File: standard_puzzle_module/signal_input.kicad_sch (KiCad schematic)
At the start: 6 parts

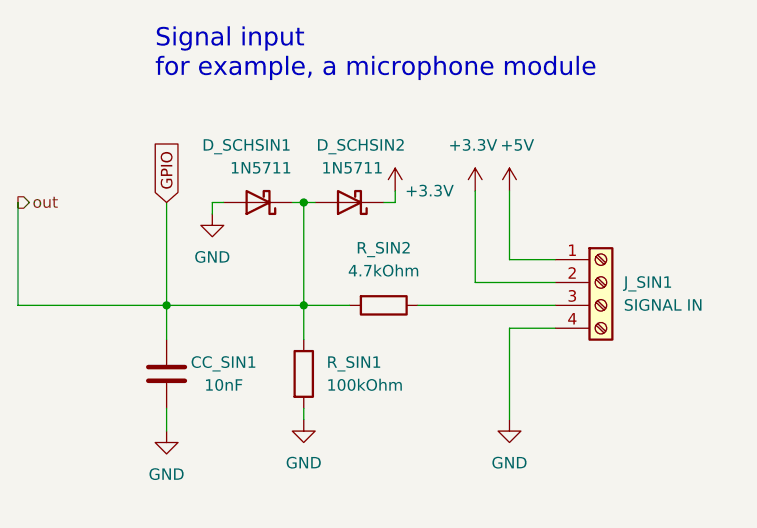
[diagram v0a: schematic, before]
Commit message: feat: dump working files before blackout
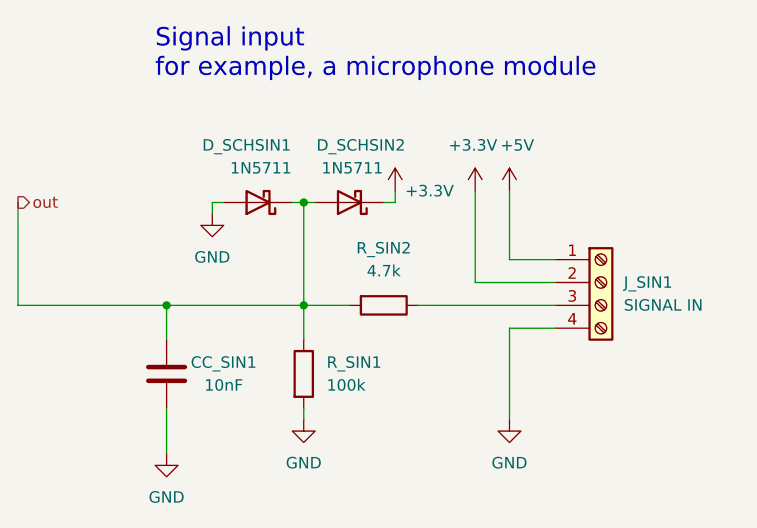
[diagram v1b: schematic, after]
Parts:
- R_SIN1: value 100kOhm -> 100k
- R_SIN2: value 4.7kOhm -> 4.7k
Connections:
- net GPIO renamed out
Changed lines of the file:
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@@
 	(wire
 		(pts
-			(xy 119.38 96.52) (xy 119.38 107.95)
+			(xy 119.38 119.38) (xy 119.38 124.46)
 		)
 		(stroke
@@
 	(wire
 		(pts
-			(xy 119.38 119.38) (xy 119.38 121.92)
-		)
-		(stroke
-			(width 0)
-			(type default)
-		)
-	)
-	(wire
-		(pts
 			(xy 157.48 110.49) (xy 157.48 120.65)
 		)
@@
 			(width 0)
 			(type default)
-		)
-	)
-	(global_label "GPIO"
-		(shape input)
-		(at 119.38 96.52 90)
-		(fields_autoplaced yes)
-		(effects
-			(font
-				(size 1.27 1.27)
-			)
-			(justify left)
-		)
-		(property "Intersheetrefs" "${INTERSHEET_REFS}"
-			(at 119.38 89.0595 90)
-			(hide yes)
-			(show_name no)
-			(do_not_autoplace no)
-			(effects
-				(font
-					(size 1.27 1.27)
-				)
-				(justify left)
-			)
 		)
 	)
@@
 			)
 		)
-		(property "Value" "4.7kOhm"
+		(property "Value" "4.7k"
 			(at 143.51 104.14 90)
 			(show_name no)
@@
 	(symbol
 		(lib_id "power:GND")
-		(at 119.38 121.92 0)
+		(at 119.38 124.46 0)
 		(unit 1)
 		(body_style 1)
@@
 		(dnp no)
 		(property "Reference" "#PWR042"
-			(at 119.38 128.27 0)
+			(at 119.38 130.81 0)
 			(hide yes)
 			(show_name no)
@@
 		)
 		(property "Value" "GND"
-			(at 119.38 126.746 0)
+			(at 119.38 129.286 0)
 			(show_name no)
 			(do_not_autoplace no)
@@
 		)
 		(property "Footprint" ""
-			(at 119.38 121.92 0)
+			(at 119.38 124.46 0)
 			(hide yes)
 			(show_name no)
@@
 		)
 		(property "Datasheet" ""
-			(at 119.38 121.92 0)
+			(at 119.38 124.46 0)
 			(hide yes)
 			(show_name no)
@@
 		)
 		(property "Description" "Power symbol creates a global label with name \"GND\" , ground"
-			(at 119.38 121.92 0)
+			(at 119.38 124.46 0)
 			(hide yes)
 			(show_name no)
@@
 			)
 		)
-		(property "Value" "100kOhm"
+		(property "Value" "100k"
 			(at 137.16 116.8399 0)
 			(show_name no)
